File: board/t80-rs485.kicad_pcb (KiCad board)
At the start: 2 copper layers, 20 x 80 mm, 20 parts, among them J2 RS485, U1 ATSAMD09C13A-SS, U2 MAX232, X1 SWD

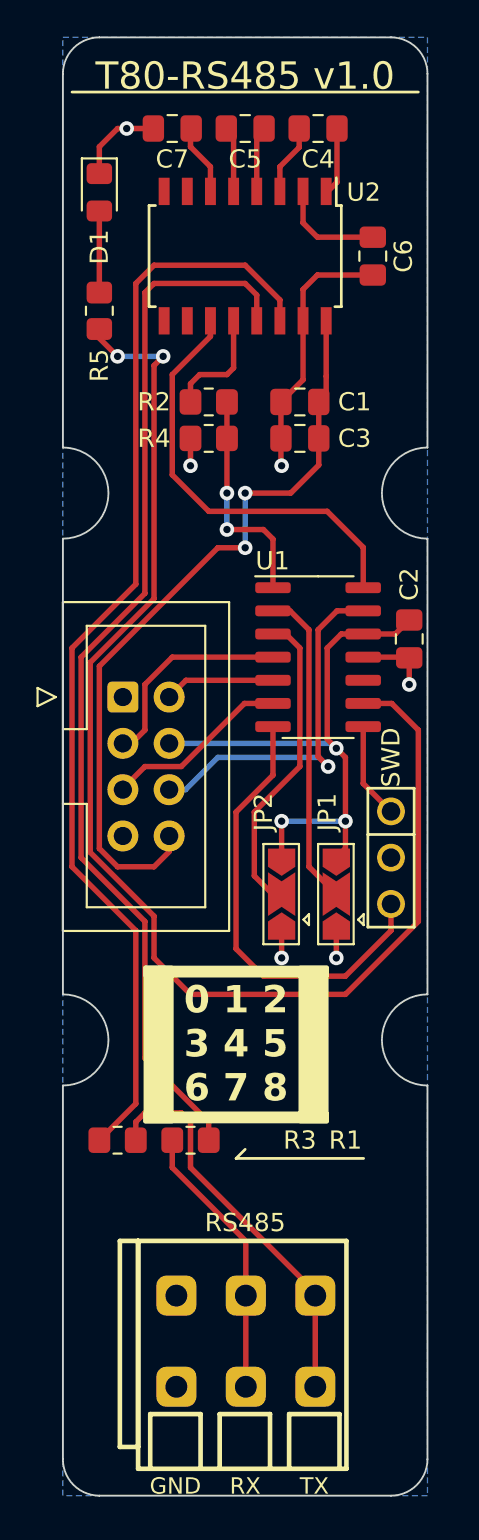
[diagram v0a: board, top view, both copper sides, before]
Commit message: WIP
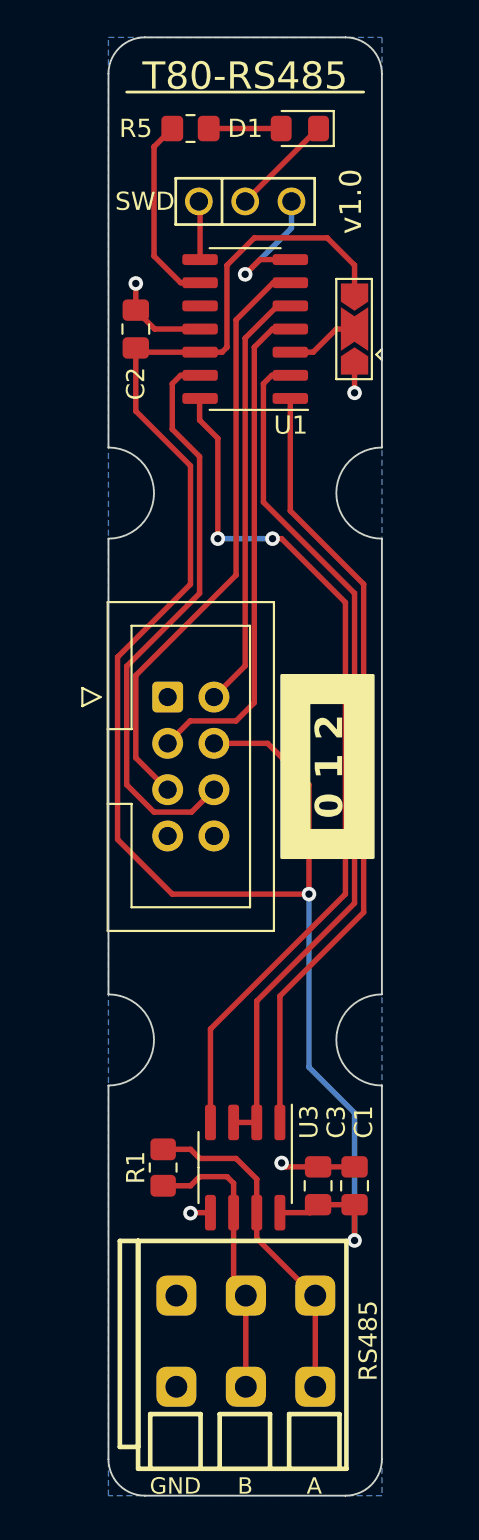
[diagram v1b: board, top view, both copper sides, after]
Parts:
- removed C4, C5, C6, C7: 1u, Capacitor_SMD:C_0805_2012Metric_Pad1.18x1.45mm_HandSolder
- removed JP2: A1, Jumper:SolderJumper-3_P2.0mm_Open_TrianglePad1.0x1.5mm
- removed R2, R3, R4: 270R, Resistor_SMD:R_0805_2012Metric_Pad1.20x1.40mm_HandSolder
- removed U2: MAX232, Package_SO:SOIC-16W_5.3x10.2mm_P1.27mm
- added U3: ST3485EBD, Package_SO:SOIC-8_3.9x4.9mm_P1.27mm, F.Cu at (128.0, 107.2)
- R1: value 270R -> 120R
- moved C1 43.1 mm to (134.0, 108.2), turned to -90 degrees
- moved C3 41.0 mm to (132.0, 108.2), turned to -90 degrees
- moved X1 36.9 mm to (128.0, 54.2), turned to 0 degrees
- moved JP1 31.0 mm to (134.0, 61.2)
- moved C2 22.7 mm to (122.0, 61.2), turned to -90 degrees
- moved U1 18.4 mm to (128.0, 61.2), turned to 180 degrees
- moved D1 11.5 mm to (131.0, 50.2), turned to 180 degrees
- moved R5 11.2 mm to (125.0, 50.2), turned to 0 degrees
- moved R1 2.92 mm to (123.5, 107.2), turned to 90 degrees
- moved X2 2.46 mm to (123.7, 81.4)
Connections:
- net /TX_RS485 renamed /RS485_B
- C1 pad 2: +5V -> +3V3
- C3 pad 2: +5V -> +3V3
- J2 pad 2: /RX_RS485 -> /RS485_A
- JP1 pad 2: /A1 -> /ADDR
- R1 pad 1: Net-(U2-T1OUT) -> /RS485_A
- U1 pad 1: /RX_3V -> /RX
- U1 pad 14: /TX_3V -> /TX
- U1 pad 2: /A1 -> /TXE
- U1 pad 3: /A2 -> /ADDR
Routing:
- net +3V3: track 32.0 -> 99.5 mm, vias 3 -> 2
- net /LED: track 71.6 -> 10.5 mm, vias 2 -> 0
- net Net-(U2-T1OUT): track 60.9 -> 0.00 mm
- net Net-(U2-R1IN): track 58.8 -> 0.00 mm
- net /TX: track 0.00 -> 48.2 mm, vias 0 -> 2
- net /TXE: track 0.00 -> 47.8 mm
- net /RX: track 0.00 -> 43.3 mm
- net +5V: track 42.0 -> 0.00 mm, vias 2 -> 0
- net /TX_3V: track 23.7 -> 0.00 mm
- net /RST: track 10.2 -> 32.6 mm
- net /SCL: track 6.08 -> 23.6 mm
- net /A1: track 17.5 -> 0.00 mm
- net /A2: track 17.2 -> 0.00 mm
- net /SWCLK: track 24.6 -> 7.86 mm, vias 0 -> 1
- net /SDA: track 11.7 -> 27.6 mm
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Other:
- board size 20 x 80 mm -> 15 x 80 mm
- board text added: "0 1 2"
- board text added: "A"
- board text added: "B"
- board text added: "T80-RS485"
- board text added: "v1.0"
- board text removed: "0 1 2 3 4 5 6 7 8"
- board text removed: "RX"
- board text removed: "T80-RS485 v1.0"
- board text removed: "TX"
